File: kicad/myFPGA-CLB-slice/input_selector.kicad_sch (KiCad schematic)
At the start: 42 parts, among them U34 74LS153, U35 74LS153, U36 74LS153, U37 74LS153

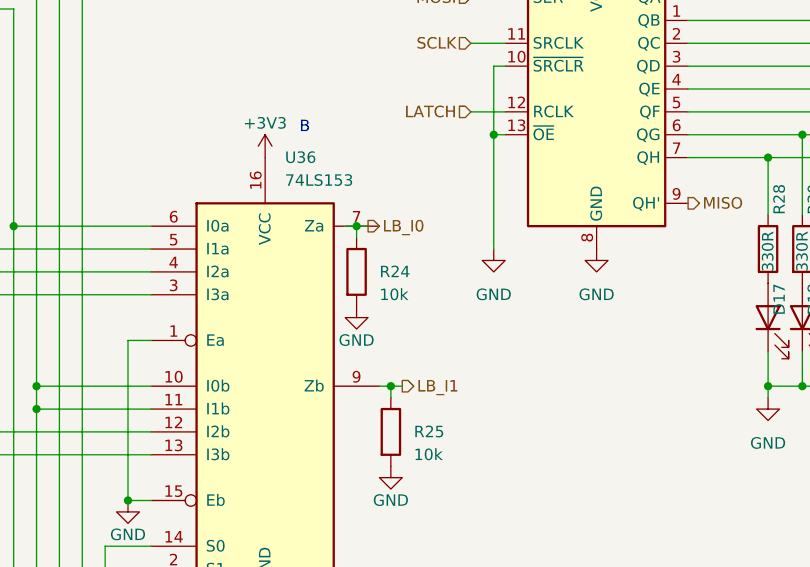
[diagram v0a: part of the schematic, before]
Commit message: progress in pcb of CLB
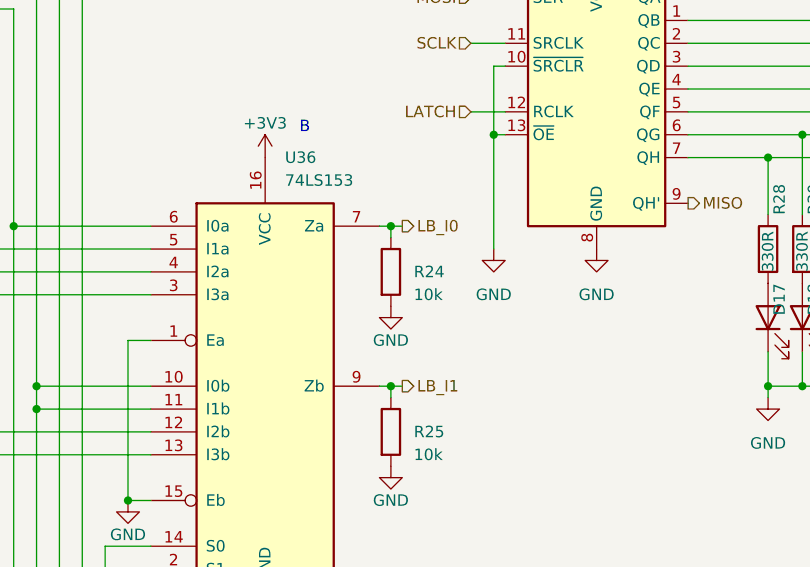
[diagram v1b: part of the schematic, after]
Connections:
- net LB_I0: now also U36.7 (Za)
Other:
- moved on the sheet: R24
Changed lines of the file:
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@@
   (junction (at 252.73 116.84) (diameter 0) (color 0 0 0 0)
   )
-  (junction (at 186.69 52.07) (diameter 0) (color 0 0 0 0)
-  )
   (junction (at 44.45 151.13) (diameter 0) (color 0 0 0 0)
   )
@@
   (junction (at 16.51 43.18) (diameter 0) (color 0 0 0 0)
   )
+  (junction (at 190.5 52.07) (diameter 0) (color 0 0 0 0)
+  )
   (junction (at 54.61 27.94) (diameter 0) (color 0 0 0 0)
   )
@@
     (stroke (width 0) (type default))
   )
+  (wire (pts (xy 190.5 52.07) (xy 191.77 52.07))
+    (stroke (width 0) (type default))
+  )
   (wire (pts (xy 110.49 43.18) (xy 110.49 120.65))
     (stroke (width 0) (type default))
@@
     (stroke (width 0) (type default))
   )
-  (wire (pts (xy 186.69 52.07) (xy 187.96 52.07))
-    (stroke (width 0) (type default))
-  )
   (wire (pts (xy 256.54 116.84) (xy 260.35 116.84))
     (stroke (width 0) (type default))
@@
     (stroke (width 0) (type default))
   )
-  (wire (pts (xy 185.42 52.07) (xy 186.69 52.07))
-    (stroke (width 0) (type default))
-  )
   (wire (pts (xy 44.45 151.13) (xy 44.45 172.72))
     (stroke (width 0) (type default))
@@
     (stroke (width 0) (type default))
   )
+  (wire (pts (xy 189.23 52.07) (xy 190.5 52.07))
+    (stroke (width 0) (type default))
+  )
   (wire (pts (xy 123.19 38.1) (xy 123.19 123.19))
     (stroke (width 0) (type default))
@@
     (stroke (width 0) (type default))
   )
-  (wire (pts (xy 186.69 53.34) (xy 186.69 52.07))
-    (stroke (width 0) (type default))
-  )
   (wire (pts (xy 46.99 30.48) (xy 46.99 148.59))
     (stroke (width 0) (type default))
@@
   )
   (wire (pts (xy 189.23 69.85) (xy 190.5 69.85))
+    (stroke (width 0) (type default))
+  )
+  (wire (pts (xy 190.5 52.07) (xy 190.5 53.34))
     (stroke (width 0) (type default))
   )
@@
     (effects (font (size 1.27 1.27)) (justify left))
   )
-  (hierarchical_label "LB_I0" (shape output) (at 187.96 52.07 0) (fields_autoplaced)
+  (hierarchical_label "LB_I0" (shape output) (at 191.77 52.07 0) (fields_autoplaced)
     (effects (font (size 1.27 1.27)) (justify left))
   )
@@
     )
   )
-  (symbol (lib_id "Device:R") (at 186.69 57.15 0) (unit 1)
-    (in_bom yes) (on_board yes) (dnp no)
-    (property "Reference" "R24" (at 189.23 57.15 0)
-      (effects (font (size 1.27 1.27)) (justify left))
-    )
-    (property "Value" "10k" (at 189.23 59.69 0)
-      (effects (font (size 1.27 1.27)) (justify left))
-    )
-    (property "Footprint" "Resistor_SMD:R_0603_1608Metric" (at 184.912 57.15 90)
-      (effects (font (size 1.27 1.27)) hide)
-    )
-    (property "Datasheet" "~" (at 186.69 57.15 0)
-      (effects (font (size 1.27 1.27)) hide)
-    )
-    (property "JLCPCB Part #" "C25804" (at 186.69 57.15 0)
-      (effects (font (size 1.27 1.27)) hide)
-    )
-    (property "Part Nr." "0603WAF1002T5E" (at 186.69 57.15 0)
-      (effects (font (size 1.27 1.27)) hide)
-    )
-    (property "Dielectric" "" (at 186.69 57.15 0)
-      (effects (font (size 1.27 1.27)) hide)
-    )
-    (property "Voltage" "" (at 186.69 57.15 0)
-      (effects (font (size 1.27 1.27)) hide)
-    )
-    (property "JLCPCB Alt #" "" (at 186.69 57.15 0)
-      (effects (font (size 1.27 1.27)) hide)
-    )
-    (property "package" "" (at 186.69 57.15 0)
+  (symbol (lib_id "Device:R") (at 190.5 57.15 0) (unit 1)
+    (in_bom yes) (on_board yes) (dnp no)
+    (property "Reference" "R24" (at 193.04 57.15 0)
+      (effects (font (size 1.27 1.27)) (justify left))
+    )
+    (property "Value" "10k" (at 193.04 59.69 0)
+      (effects (font (size 1.27 1.27)) (justify left))
+    )
+    (property "Footprint" "Resistor_SMD:R_0603_1608Metric" (at 188.722 57.15 90)
+      (effects (font (size 1.27 1.27)) hide)
+    )
+    (property "Datasheet" "~" (at 190.5 57.15 0)
+      (effects (font (size 1.27 1.27)) hide)
+    )
+    (property "JLCPCB Part #" "C25804" (at 190.5 57.15 0)
+      (effects (font (size 1.27 1.27)) hide)
+    )
+    (property "Part Nr." "0603WAF1002T5E" (at 190.5 57.15 0)
+      (effects (font (size 1.27 1.27)) hide)
+    )
+    (property "Dielectric" "" (at 190.5 57.15 0)
+      (effects (font (size 1.27 1.27)) hide)
+    )
+    (property "Voltage" "" (at 190.5 57.15 0)
+      (effects (font (size 1.27 1.27)) hide)
+    )
+    (property "JLCPCB Alt #" "" (at 190.5 57.15 0)
+      (effects (font (size 1.27 1.27)) hide)
+    )
+    (property "package" "" (at 190.5 57.15 0)
       (effects (font (size 1.27 1.27)) hide)
     )
@@
     )
   )
-  (symbol (lib_id "power:GND") (at 186.69 60.96 0) (unit 1)
-    (in_bom yes) (on_board yes) (dnp no)
-    (property "Reference" "#PWR?" (at 186.69 67.31 0)
-      (effects (font (size 1.27 1.27)) hide)
-    )
-    (property "Value" "GND" (at 186.69 64.77 0)
+  (symbol (lib_id "power:GND") (at 190.5 60.96 0) (unit 1)
+    (in_bom yes) (on_board yes) (dnp no)
+    (property "Reference" "#PWR?" (at 190.5 67.31 0)
+      (effects (font (size 1.27 1.27)) hide)
+    )
+    (property "Value" "GND" (at 190.5 64.77 0)
       (effects (font (size 1.27 1.27)))
     )
-    (property "Footprint" "" (at 186.69 60.96 0)
-      (effects (font (size 1.27 1.27)) hide)
-    )
-    (property "Datasheet" "" (at 186.69 60.96 0)
-      (effects (font (size 1.27 1.27)) hide)
-    )
+    (property "Footprint" "" (at 190.5 60.96 0)
+      (effects (font (size 1.27 1.27)) hide)
+    )
+    (property "Datasheet" "" (at 190.5 60.96 0)
+      (effects (font (size 1.27 1.27)) hide)
+    )
